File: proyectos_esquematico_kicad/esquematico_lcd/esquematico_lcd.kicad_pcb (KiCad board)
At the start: 2 copper layers, 2 parts, among them J1 Conn_01x14_Male, U1 RC1602A

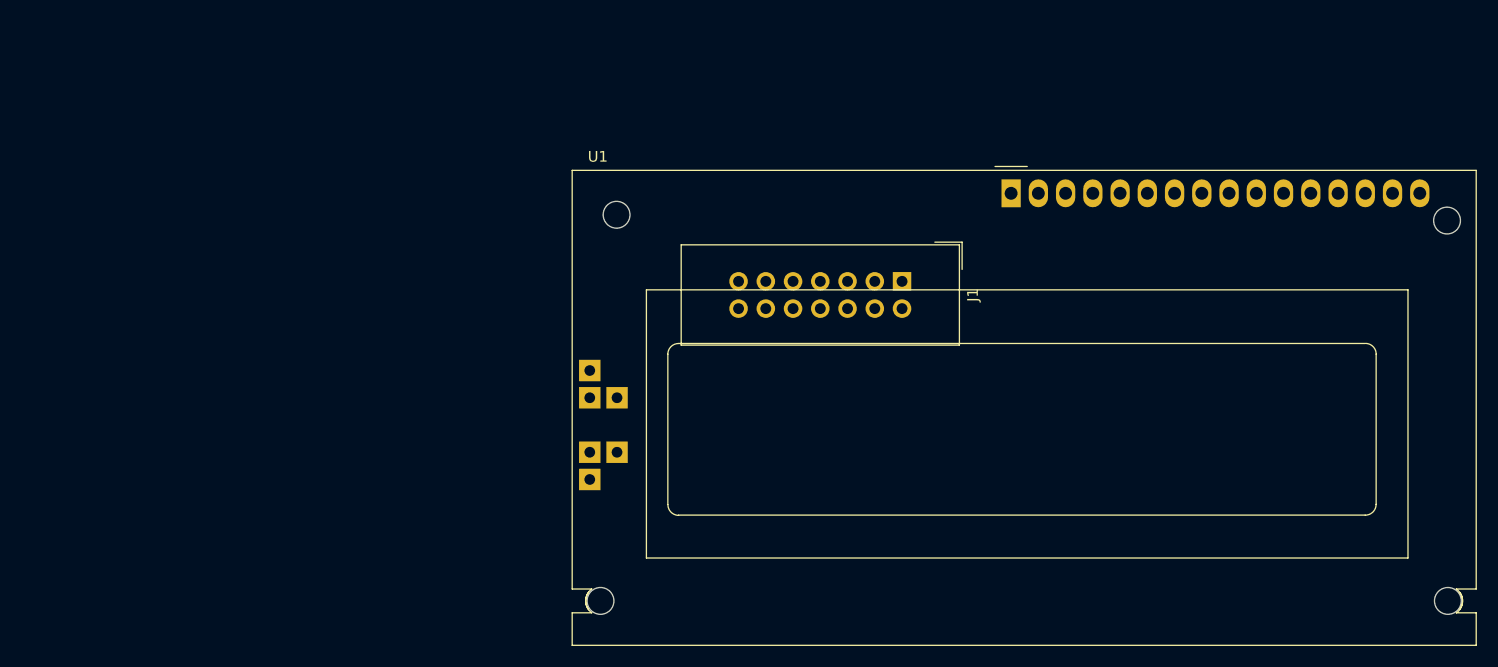
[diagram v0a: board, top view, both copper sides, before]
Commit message: Se agrega routeo LCD PCB
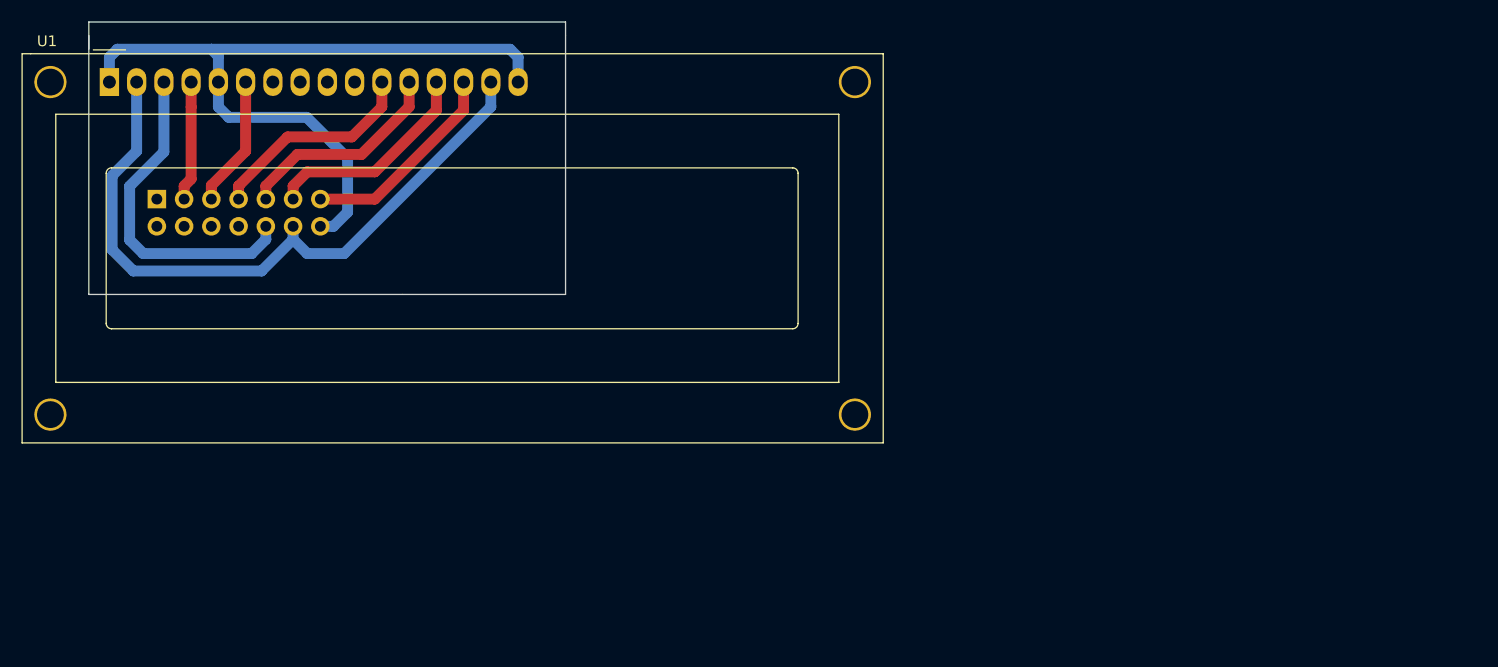
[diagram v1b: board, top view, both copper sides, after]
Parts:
- J1: moved to B.Cu
- U1: footprint Displays:RC1602A -> Display:WC1602A
- moved U1 84.7 mm to (109.9, 51.3)
- moved J1 69.9 mm to (114.3, 62.2)
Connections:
- J1 pad 1: RS -> Net-(J1-Pad1)
- J1 pad 10: DB6 -> POT
- J1 pad 11: DB7 -> DB6
- J1 pad 12: Net-(J1-Pad12) -> VCC
- J1 pad 13: VCC -> DB7
- J1 pad 3: E -> RS
- J1 pad 5: Net-(J1-Pad5) -> E
- J1 pad 7: POT -> DB4
- J1 pad 8: DB4 -> Net-(J1-Pad8)
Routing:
- net GND: track 0.00 -> 71.1 mm
- net VCC: track 0.00 -> 63.7 mm
- net POT: track 0.00 -> 31.0 mm
- net DB6: track 0.00 -> 20.1 mm
- net DB5: track 0.00 -> 19.9 mm
- net DB4: track 0.00 -> 19.9 mm
- net DB7: track 0.00 -> 19.4 mm
- net E: track 0.00 -> 12.2 mm
- net RS: track 0.00 -> 11.2 mm
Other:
- board outline added: 44.5 x 25.4 mm
- rule pad_to_mask_clearance: 0.051 -> 0
- rule trace_min: 0.4064 -> 0.2
